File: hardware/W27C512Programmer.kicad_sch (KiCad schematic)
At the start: 114 parts, among them J1 CTRL, J2 MSB, J3 LSB, J4 Ext_UART, J5 OLED, J6 VP, J7 SAO, Q1 MMBT3904, Q10 MMBT3906, Q11 MMBT3904, Q12 MMBT3906, Q2 MMBT3906, Q3 MMBT3904, Q4 MMBT3904, Q5 MMBT3904, Q6 MMBT3906, Q7 MMBT3906, Q8 MMBT3906, Q9 MMBT3904, SW1 RST, SW2 USR, U1 MIC2288, U2 74HC573, U3 74HC573, U4 74HC573, U5 28/32 pin ROM

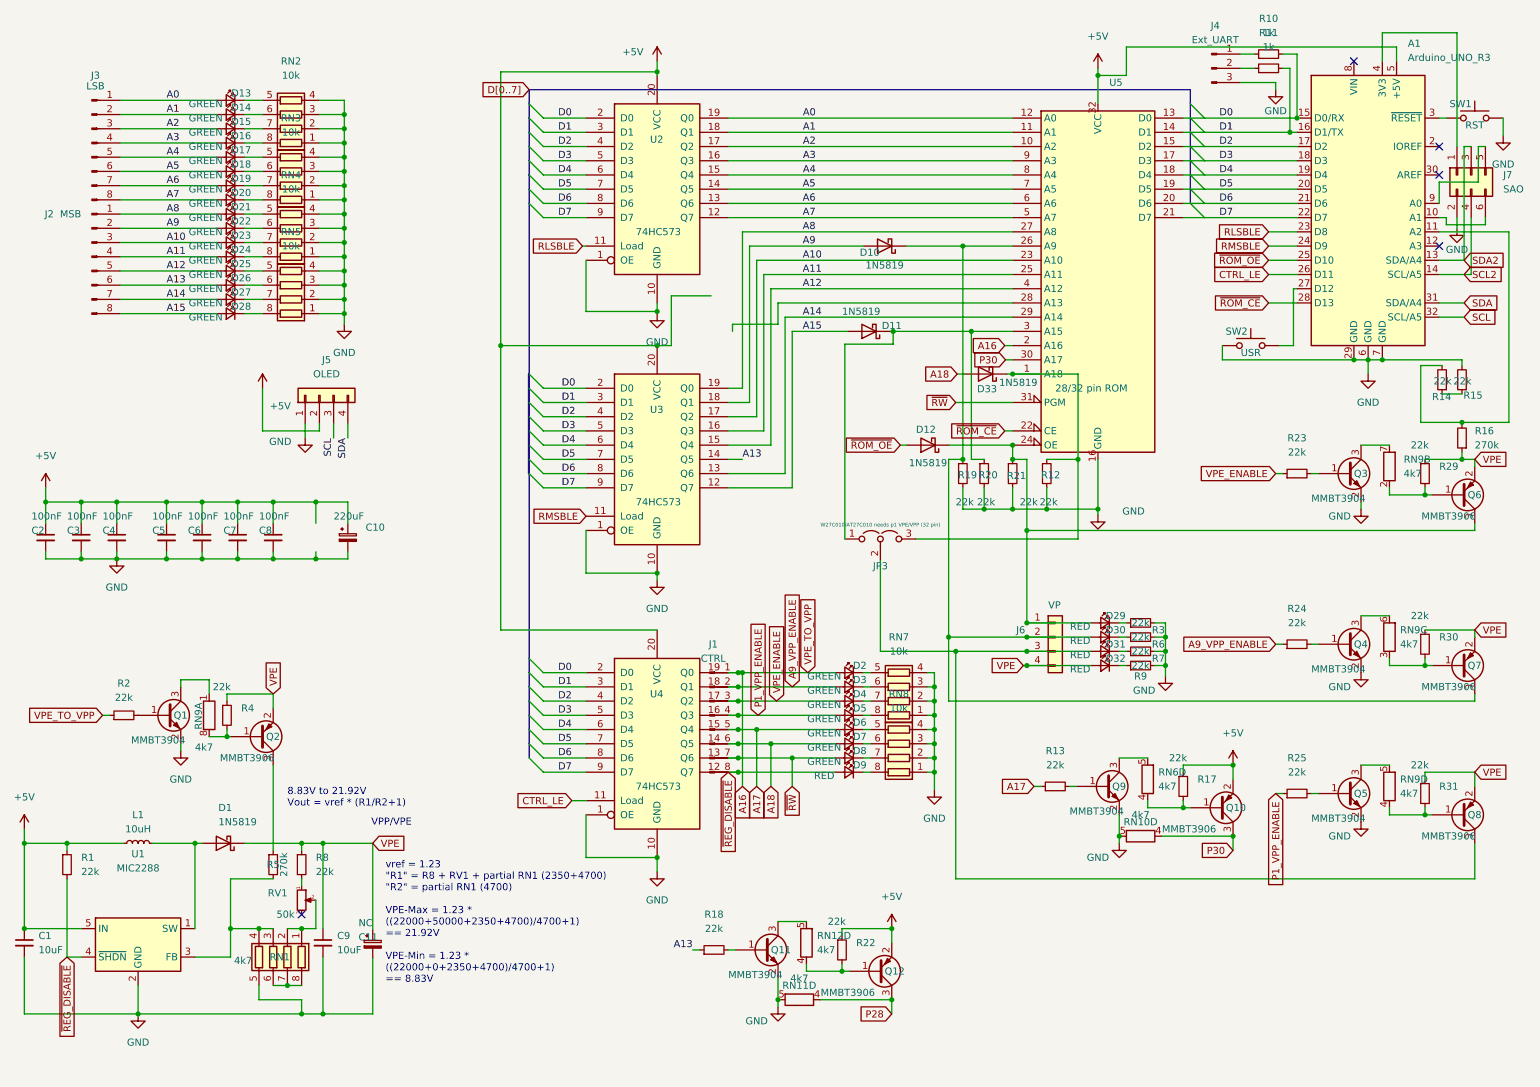
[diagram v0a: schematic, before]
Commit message: Rev2
Hopefully this does what it's supposed to...
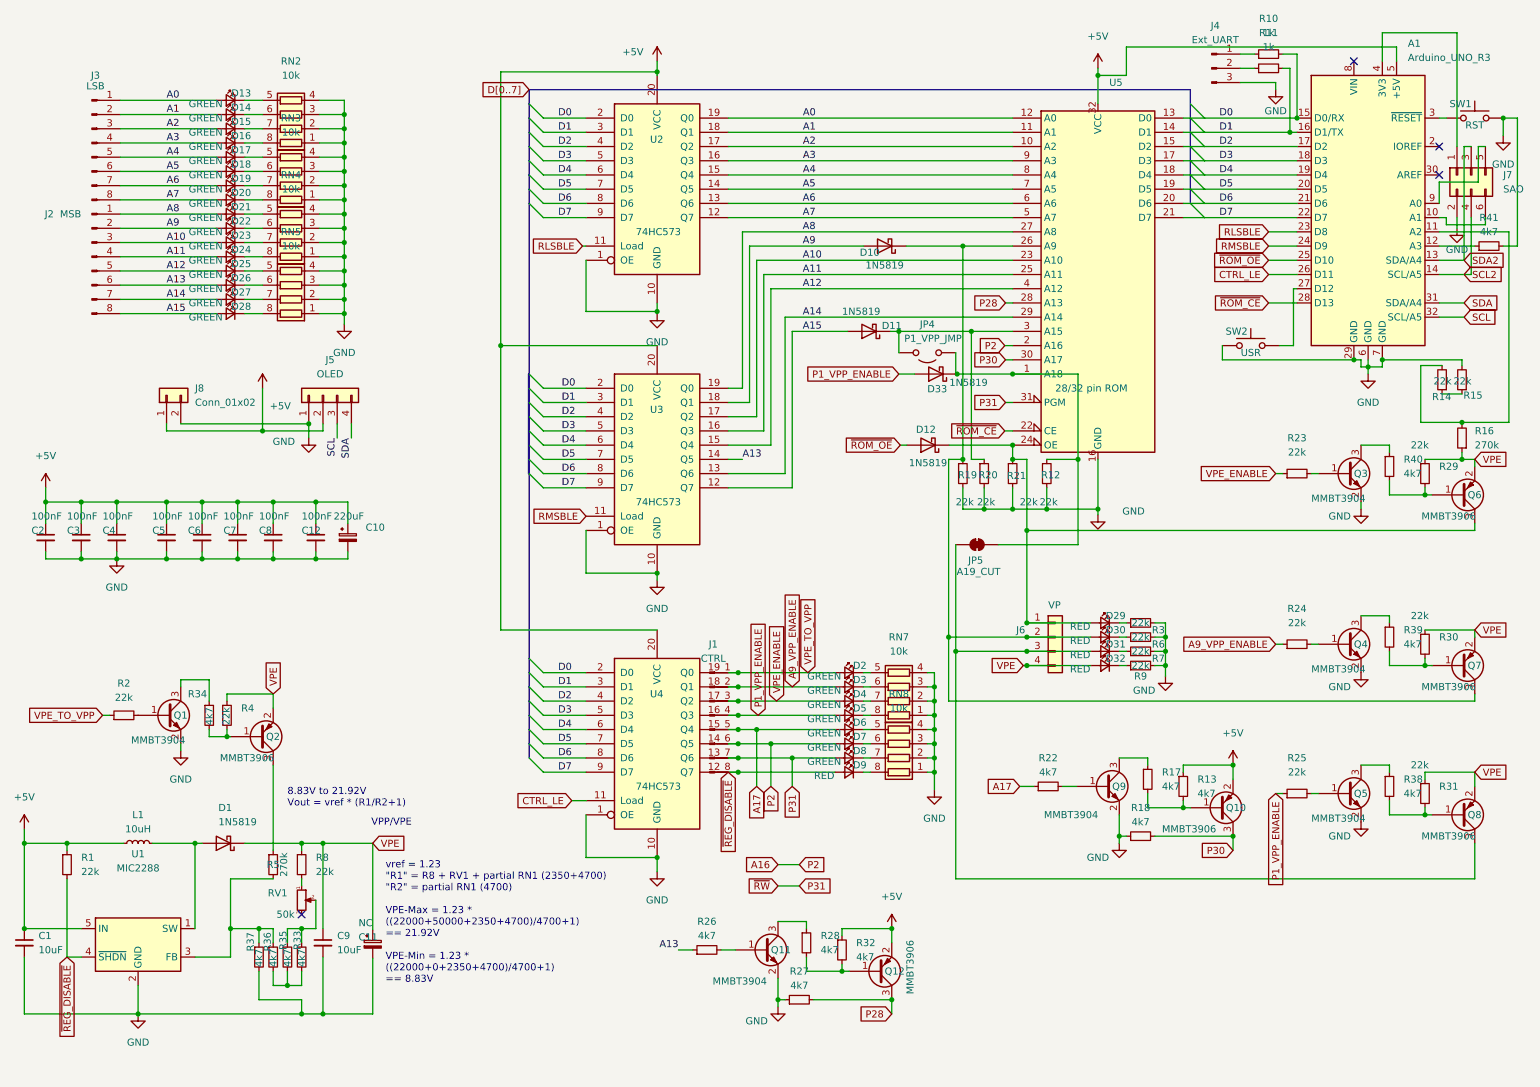
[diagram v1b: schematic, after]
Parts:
- removed JP3: W27C010/AT27C010 needs p1 VPE/VPP (32 pin), Jumper:SolderJumper-3_P1.3mm_Open_RoundedPad1.0x1.5mm, symbol Jumper:Jumper_3_Open
- removed RN1: 4k7, Resistor_SMD:R_Array_Convex_4x0603, symbol Device:R_Pack04
- removed RN10, RN11, RN12, RN6, RN9: 4k7, Resistor_SMD:R_Array_Convex_4x0603, symbol Device:R_Pack04_Split
- added C12: 100nF, Capacitor_SMD:C_0603_1608Metric, symbol Device:C_Small
- added J8: Conn_01x02, Connector_PinHeader_2.54mm:PinHeader_1x02_P2.54mm_Vertical, symbol Connector_Generic:Conn_01x02
- added JP4: P1_VPP_JMP, Connector_PinHeader_2.54mm:PinHeader_1x02_P2.54mm_Vertical, symbol Jumper:Jumper_2_Open
- added JP5: A19_CUT, Jumper:SolderJumper-2_P1.3mm_Bridged_RoundedPad1.0x1.5mm, symbol Jumper:SolderJumper_2_Bridged
- added R26, R27, R28, R32, R33, R34, R35, R36, R37, R38, R39, R40, R41: 4k7, Resistor_SMD:R_0402_1005Metric, symbol Device:R_Small
- R13, R17, R18, R22: value 22k -> 4k7; footprint Resistor_SMD:R_0603_1608Metric -> Resistor_SMD:R_0402_1005Metric; LCSC (none) -> C25900
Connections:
- net +5V: now also R13.1, C12.1, J8.1 (Pin_1), R32.1; no longer R17.1, R22.1
- net A13: now also R26.1; no longer R18.1
- net A16: now also D7.2 (A), J1.6 (Pin_6), U4.14 (Q5); no longer D2.2 (A), J1.1 (Pin_1), R2.1, U4.19 (Q0)
- net A17: now also R22.1; no longer R13.1
- net GND: now also R18.1, C12.2, J8.2 (Pin_2), R27.1, R37.2, R41.2
- net P1_VPP_ENABLE: now also D33.2 (A)
- net P28: now also U5.28 (A13), R27.2
- net P30: now also R18.2
- net at D11.1 (K), R20.1, U5.3 (A15): now also JP4.2 (B)
- net at D31.2 (A), J6.3 (Pin_3), Q8.3 (C): now also JP5.1 (A)
- net at Q1.3 (C): now also R34.1
- net at Q2.1 (B), R4.2: now also R34.2
- net at R5.2, U1.3 (FB): now also R36.1, R37.1
- net at Q7.1 (B), R30.2: now also R39.2
- net at Q12.1 (B): now also R28.2, R32.2; no longer R22.2
- net at Q11.3 (C): now also R28.1
- net at Q4.3 (C): now also R39.1
- net at Q8.1 (B), R31.2: now also R38.2
- net at Q5.3 (C): now also R38.1
- net at Q6.1 (B), R29.2: now also R40.2
- net at Q3.3 (C): now also R40.1
- net at R13.2: now also Q10.1 (B), R17.2; no longer Q9.1 (B)
- net at Q9.3 (C): now also R17.1
- net at RV1.2: now also R33.1, R35.1
- net at Q11.1 (B): now also R26.2; no longer R18.2
- net at D33.1 (K), R12.1, U5.1 (A18): now also JP4.1 (A), JP5.2 (B)
- net at A1.12 (A3): now also R41.1
- removed net A18: D33.2 (A), D7.2 (A), J1.6 (Pin_6), U4.14 (Q5)
- net ~{RW} renamed P31
- new net: R33.2, R35.2, R36.2
- new net: Q9.1 (B), R22.2
- new net VPE_TO_VPP: D2.2 (A), J1.1 (Pin_1), R2.1, U4.19 (Q0)
- no-connect marks 5 -> 4
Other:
- moved on the sheet: D33, J5
